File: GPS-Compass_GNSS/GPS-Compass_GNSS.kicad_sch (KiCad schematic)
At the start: 36 parts, among them J1 SMA_F, J2 Conn_01x10_Socket, Q1 BC337, SW1 GNSS_RST, U1 BGA725L6E6327FTSA1, U2 TESEO-LIV3R

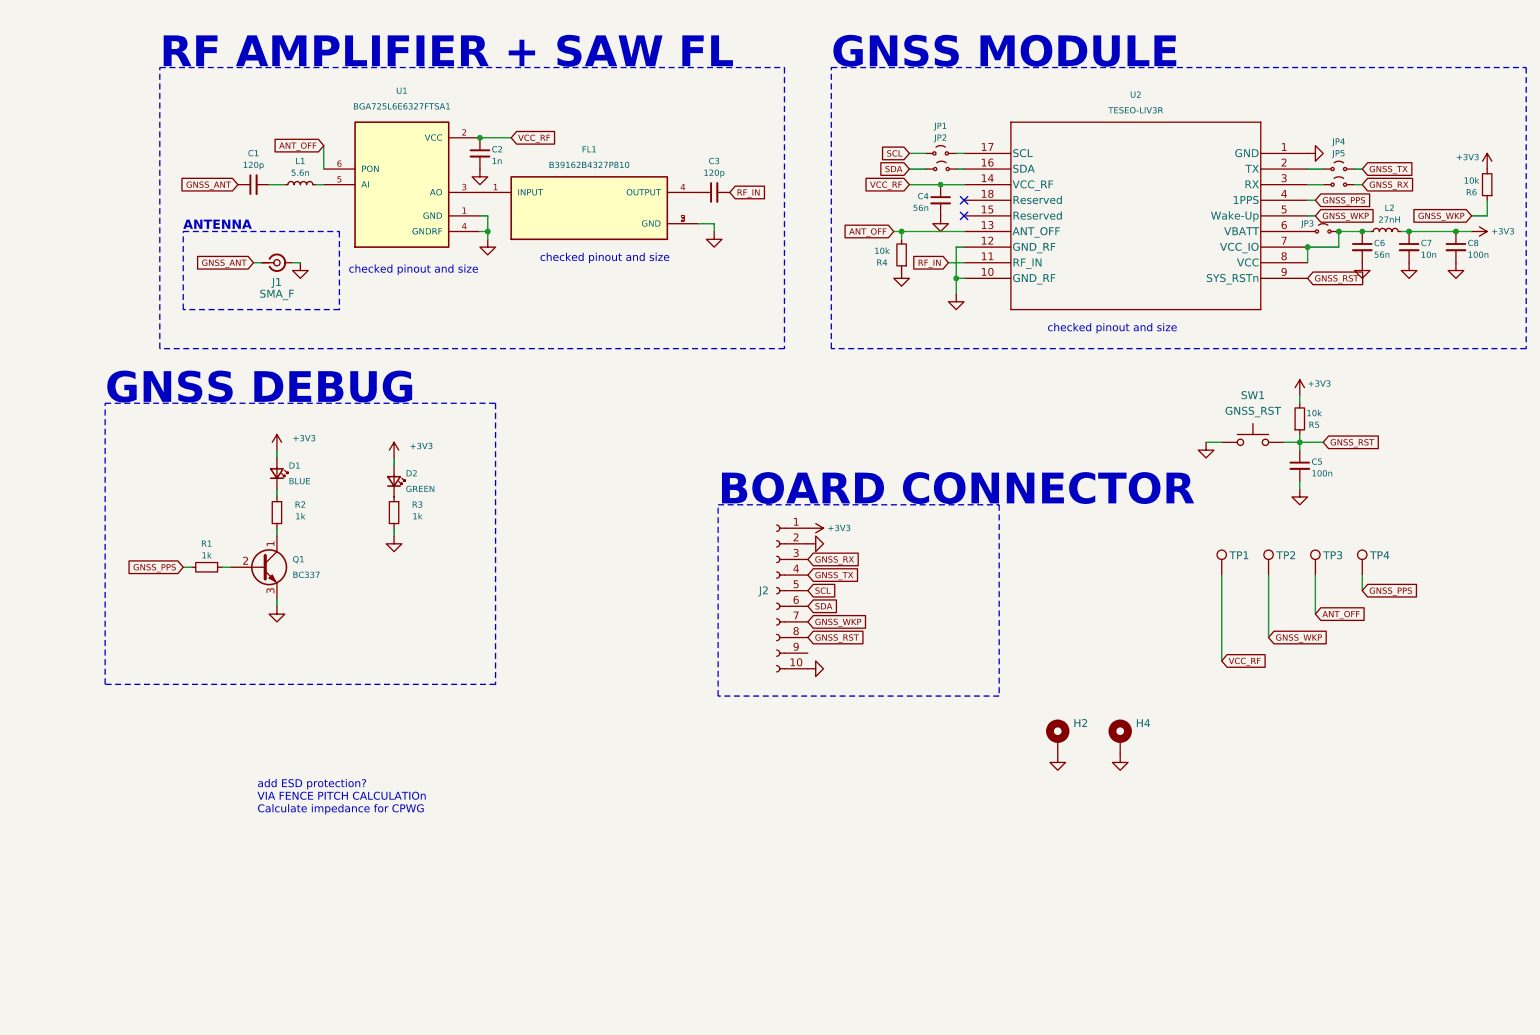
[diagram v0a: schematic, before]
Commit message: finished
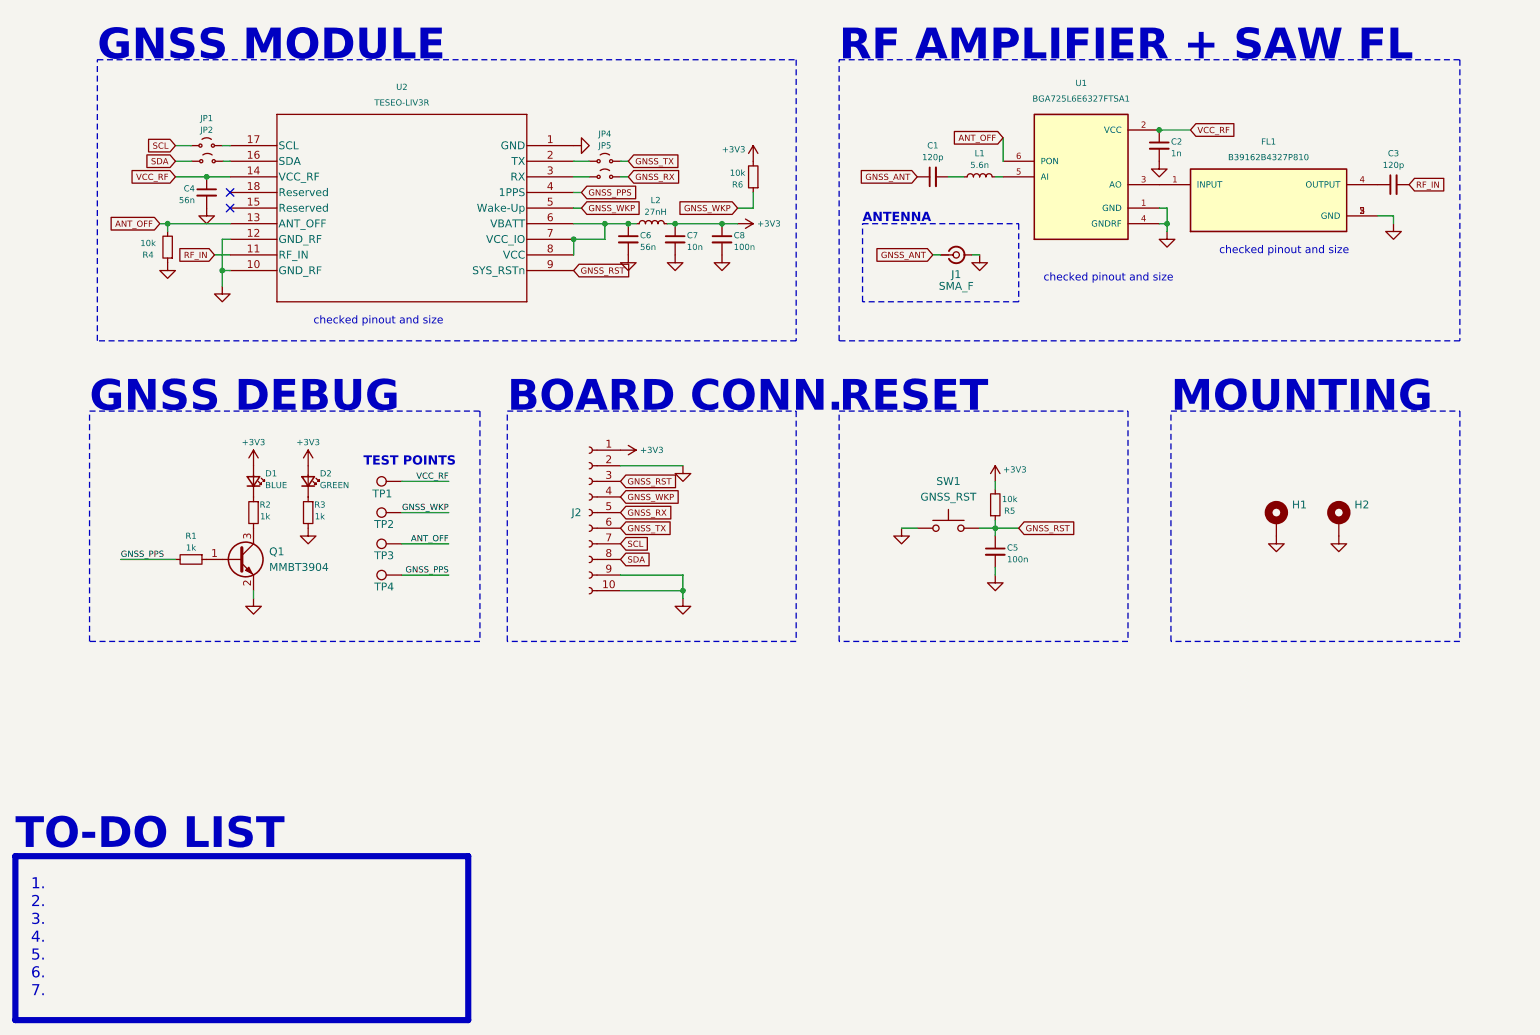
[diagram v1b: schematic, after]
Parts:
- removed JP3: Jumper_2_Small_Open, Jumper:SolderJumper-2_P1.3mm_Open_RoundedPad1.0x1.5mm, symbol Jumper:Jumper_2_Small_Open
- removed Q1: BC337, Package_TO_SOT_THT:TO-92_Inline, symbol Transistor_BJT:BC337
- added Q1: MMBT3904, Package_TO_SOT_SMD:SOT-23, symbol Transistor_BJT:MMBT3904
- renumbered H2 to H1, H4 to H2
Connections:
- net GND: now also J2.9 (Pin_9), Q1.2 (E)
- net GNSS_RST: now also J2.3 (Pin_3); no longer J2.8 (Pin_8)
- net GNSS_RX: now also J2.5 (Pin_5); no longer J2.3 (Pin_3)
- net GNSS_TX: now also J2.6 (Pin_6); no longer J2.4 (Pin_4)
- net GNSS_WKP: now also J2.4 (Pin_4); no longer J2.7 (Pin_7)
- net SCL: now also J2.7 (Pin_7); no longer J2.5 (Pin_5)
- net SDA: now also J2.8 (Pin_8); no longer J2.6 (Pin_6)
- net at C6.1, L2.2, U2.7 (VCC_IO)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: now also U2.6 (VBATT)
- net at R2.2: now also Q1.3 (C)
- net at R1.1: now also Q1.1 (B)
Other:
- note added: "1. 2. 3. 4. 5. 6. 7."
- note added: "BOARD CONN."
- note added: "MOUNTING"
- note added: "RESET"
- note added: "TEST POINTS"
- note added: "TO-DO LIST"
- note removed: "BOARD CONNECTOR"
- note removed: "add ESD protection? VIA FENCE PITCH CALCULATIOn Calculate impedance for CPWG"
- company: (none) -> SPS na Proseku
- title: (none) -> GNSS_Module
- moved on the sheet: C1, C2, C3, C4, C5, C6, C7, C8, D1, D2, FL1, H1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
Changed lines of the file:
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@@
 	(generator_version "9.0")
 	(paper "A4")
+	(title_block
+		(title "GNSS_Module")
+		(date "2025-08-26")
+		(rev "v1.0.0")
+		(company "SPS na Proseku")
+		(comment 1 "made by bismarx")
+		(comment 2 "GNSS module for GPS Compass project")
+	)
